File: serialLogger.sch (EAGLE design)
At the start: 11 parts

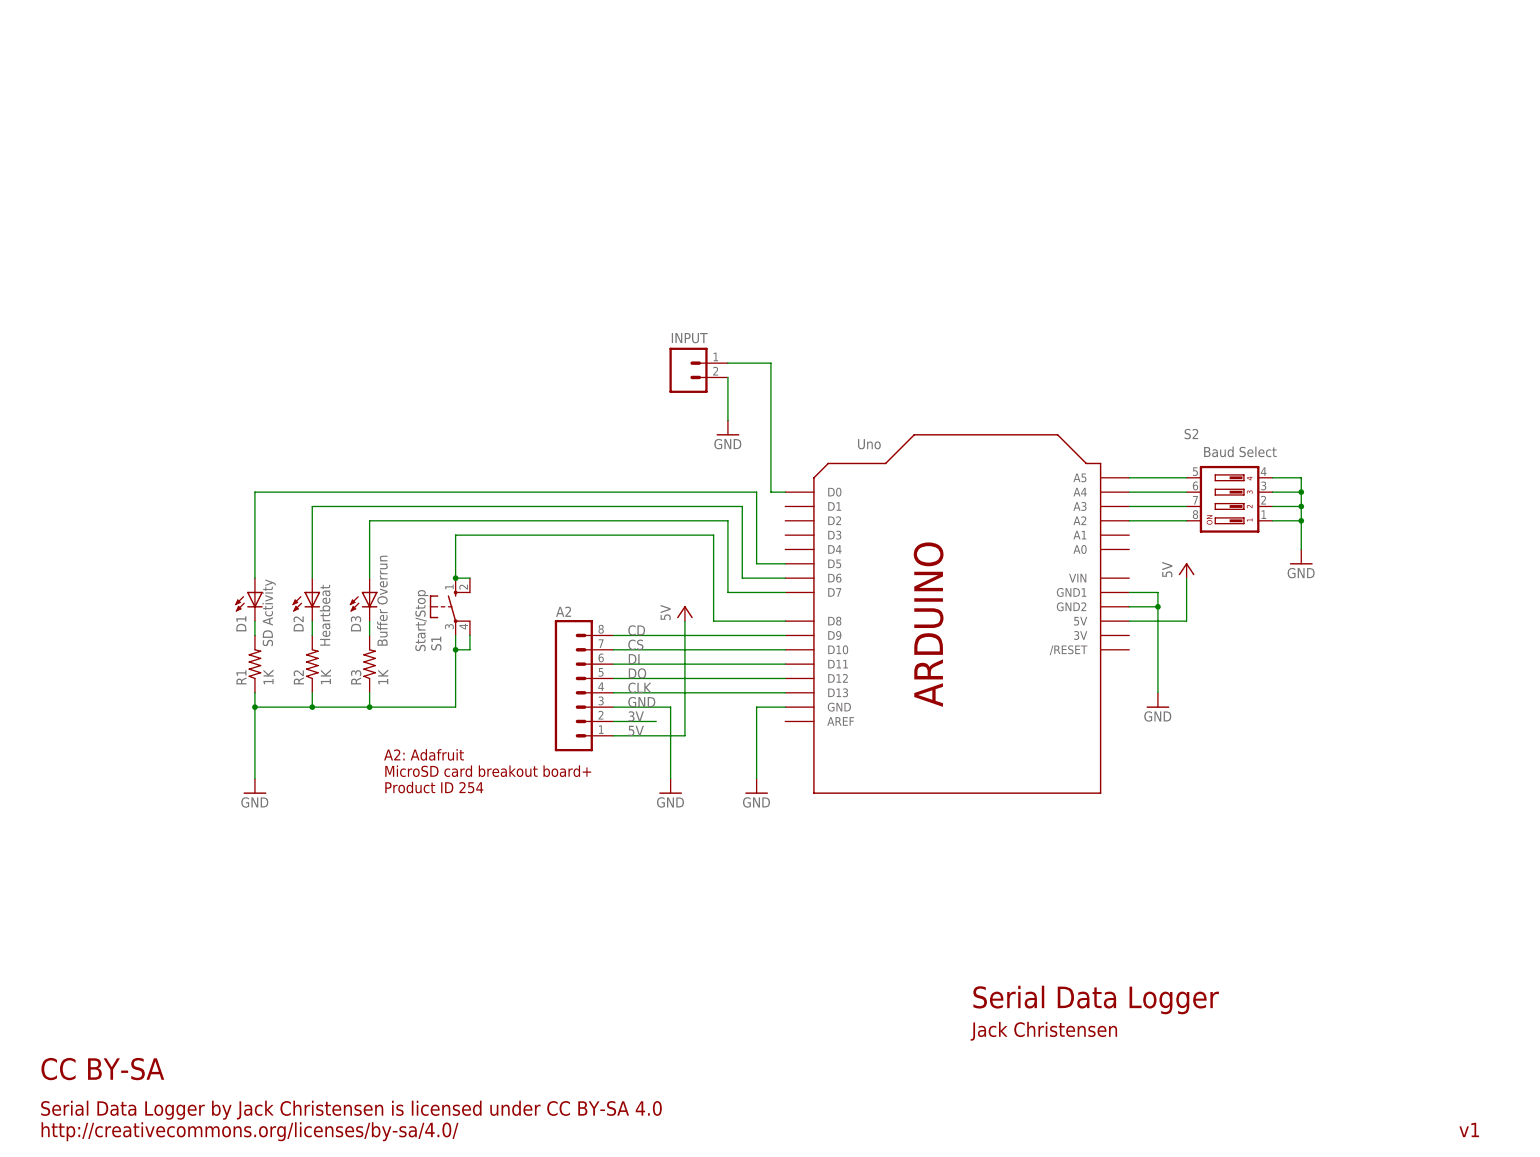
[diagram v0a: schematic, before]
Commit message: Initial v2 board.
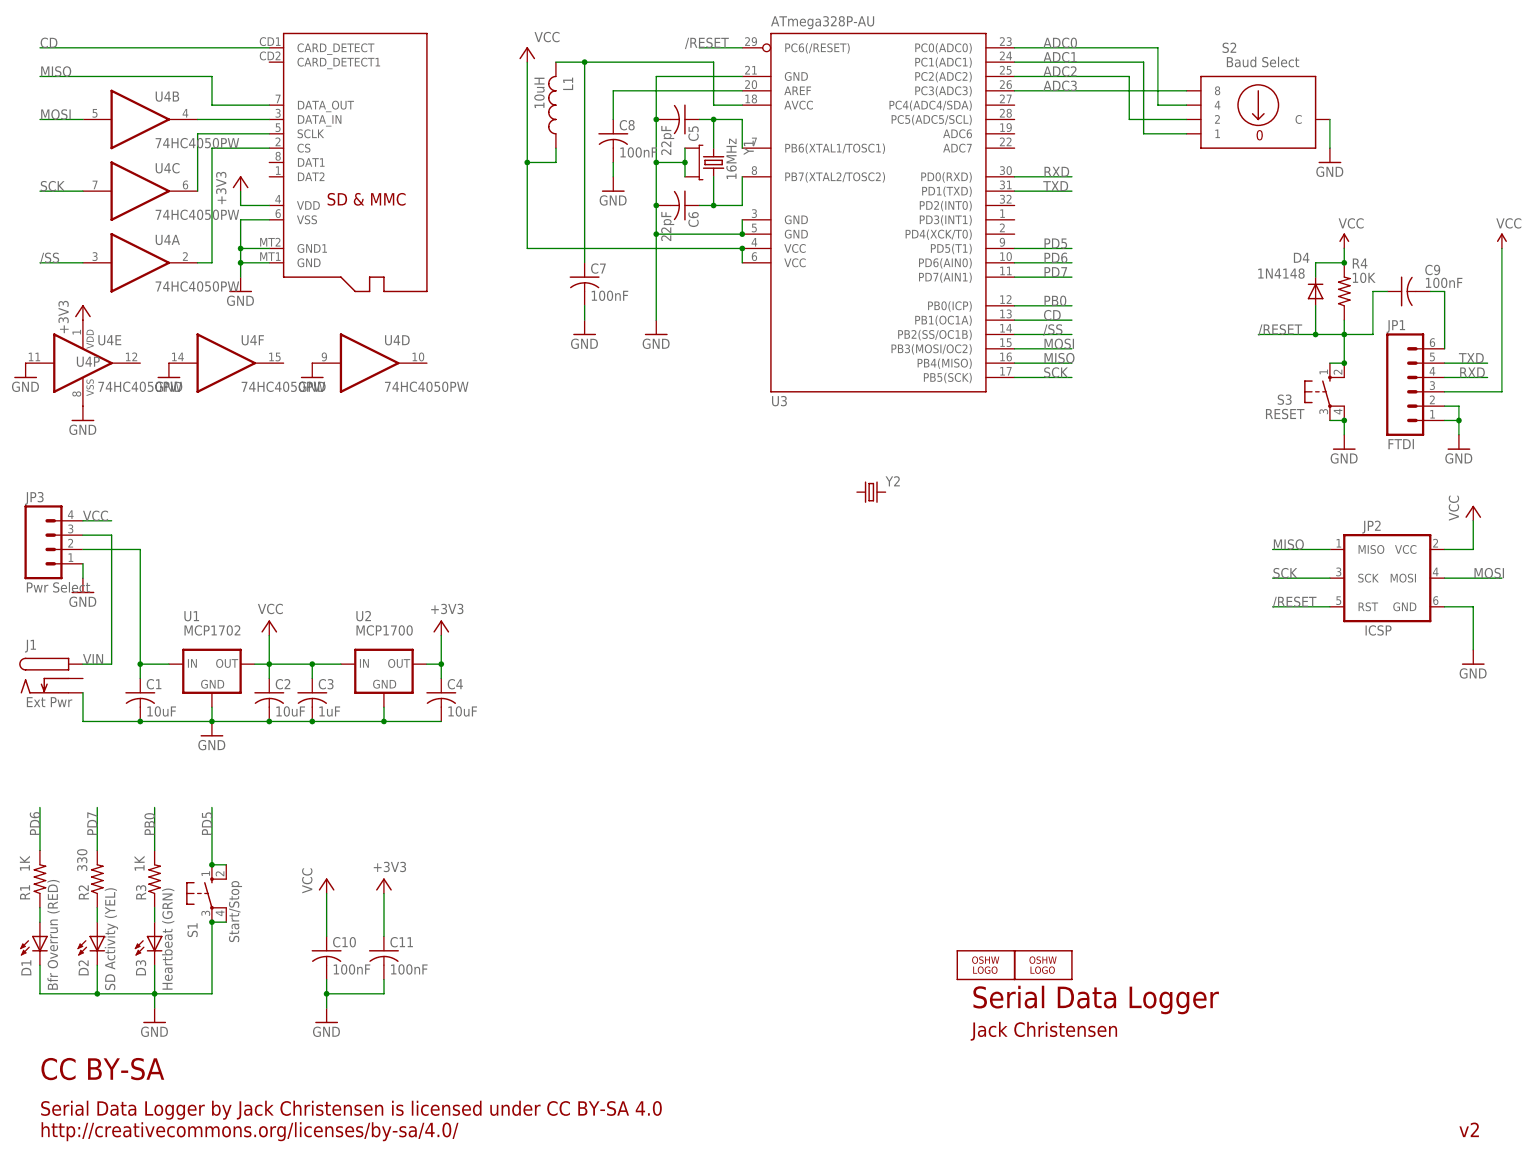
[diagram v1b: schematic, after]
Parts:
- removed A1: UNO, adafruit:ARDUINOUNO
- removed A2: (no value), SparkFun:M08LOCK
- removed INPUT: (no value), SparkFun:M02
- added C1, C2, C4: 10uF, _jc:C-USM0805
- added C10, C11, C7, C8, C9: 100nF, _jc:C-USM0805
- added C3: 1uF, _jc:C-USM0805
- added C5, C6: 22pF, _jc:C-USM0805
- added D4: 1N4148, _jc:DIODESOD-323F-A
- added J1: Ext Pwr, _jc:POWER-JACK
- added JP1: FTDI, SparkFun:M06LOCK
- added JP2: ICSP, _jc:AVR_SPI_PRG_62X3_LOCK
- added JP3: Pwr Select, SparkFun:M04LOCK
- added L1: 10uH, _jc:INDUCTORM0805
- added LOGO1, LOGO2: OSHW_LOGO_10MILX0200-NT, ohw-logo:OSHW_LOGO_10MILX0200-NT
- added R4: 10K, _jc:R-US_M0805
- added S3: RESET, _jc:10-XXOCT
- added U1: MCP1702, _jc:MCP1700SOT89
- added U2: MCP1700, _jc:MCP1700SOT23
- added U3: ATmega328P-AU, atmel:MEGA8-AI
- added U4: 74HC4050PW, 40xx:4050PW
- added X1: MICROSD, adafruit:MICROSD
- added Y1: 16MHz, _jc:CRYSTAL-2GNDTSX3225
- added Y2: (no value), _jc:CRYSTALABM2
- D1: value SD Activity -> Bfr Overrun (RED); device _jc:LED5MM -> _jc:LEDCHIPLED_1206
- D2: value Heartbeat -> SD Activity (YEL); device _jc:LED5MM -> _jc:LEDCHIPLED_1206
- D3: value Buffer Overrun -> Heartbeat (GRN); device _jc:LED5MM -> _jc:LEDCHIPLED_1206
- R2: value 1K -> 330
- S2: device switch-dil:219-04 -> _jc:OMRON-A6RS-102
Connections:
- removed net 3V: A2.2
- removed net 5V: A1.5V, A2.1
- removed net CLK: A1.D13, A2.4
- removed net CS: A1.D10, A2.7
- removed net DI: A1.D11, A2.6
- removed net DO: A1.D12, A2.5
- removed net N$11: A1.D5, D1.A
- removed net N$12: A1.D6, D2.A
- removed net N$13: A1.D7, D3.A
- removed net N$14: A1.D8, S1.S, S1.S1
- removed net N$5: A1.A3, S2.7
- removed net N$6: A1.A2, S2.8
- removed net N$7: D2.C, R2.2
- removed net N$8: D3.C, R3.2
- new net +3V3: C11.1, C4.1, U2.OUT, U4P.VDD, X1.VDD
- new net /RESET: C9.1, D4.A, JP2.RST, R4.1, S3.S, S3.S1, U3.PC6(/RESET)
- new net /SS: U3.PB2(SS/OC1B), U4A.I
- new net ADC0: S2.4, U3.PC0(ADC0)
- new net ADC1: S2.1, U3.PC1(ADC1)
- new net ADC2: S2.2, U3.PC2(ADC2)
- new net ADC3: S2.8, U3.PC3(ADC3)
- new net MISO: JP2.MISO, U3.PB4(MISO), X1.DATA_OUT
- new net MOSI: JP2.MOSI, U3.PB3(MOSI/OC2), U4B.I
- new net N$10: U4C.O, X1.SCLK
- new net N$15: U4A.O, X1.CS
- new net N$17: U4B.O, X1.DATA_IN
- new net N$18: C5.1, U3.PB6(XTAL1/TOSC1), Y1.1
- new net N$19: C6.1, U3.PB7(XTAL2/TOSC2), Y1.3
- new net N$20: C8.1, U3.AREF
- new net N$37: C7.1, L1.2, U3.AVCC
- new net PB0: R3.2, U3.PB0(ICP)
- new net PD5: S1.S, S1.S1, U3.PD5(T1)
- new net PD6: R1.2, U3.PD6(AIN0)
- new net PD7: R2.2, U3.PD7(AIN1)
- new net RST: C9.2, JP1.6
- new net RXD: JP1.4, U3.PD0(RXD)
- new net SCK: JP2.SCK, U3.PB5(SCK), U4C.I
- new net TXD: JP1.5, U3.PD1(TXD)
- new net VCC: C10.1, C2.1, C3.1, D4.K, JP1.3, JP2.VCC, JP3.4, L1.1, R4.2, U1.OUT, U2.IN, U3.VCC@1, U3.VCC@2
- new net VIN: J1.P$1, JP3.3
- net CD: now also U3.PB1(OC1A), X1.CARD_DETECT; no longer A1.D9, A2.8
- net GND: now also C1.2, C10.2, C11.2, C2.2, C3.2, C4.2, C5.2, C6.2, C7.2, C8.2, D1.C, D2.C, D3.C, J1.P$2, JP1.1, JP1.2, JP2.GND, JP3.1, S2.C, S3.P, S3.P1, U1.GND, U2.GND, U3.GND, U3.GND@1, U3.GND@2, U4D.I, U4E.I, U4F.I, U4P.VSS, X1.GND, X1.GND1, X1.VSS, Y1.2, Y1.4; no longer A1.GND, A1.GND1, A1.GND2, A2.3, INPUT.2, R1.1, R2.1, R3.1, S2.1, S2.2, S2.3, S2.4
- net N$1: now also D3.A, R3.1; no longer A1.D0, INPUT.1
- net N$2: now also D2.A, R2.1; no longer A1.A5, S2.5
- net N$3: now also D1.A, R1.1; no longer D1.C, R1.2
- net N$4: now also C1.1, JP3.2, U1.IN; no longer A1.A4, S2.6
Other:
- note added: "v2"
- note removed: "A2: Adafruit MicroSD card breakout board+ Product ID 254"
- note removed: "Uno"
- note removed: "v1"
- moved on the sheet: D1, D2, D3, R1, R2, R3, S1
